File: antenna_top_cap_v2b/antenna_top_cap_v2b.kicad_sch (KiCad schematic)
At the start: 32 parts, among them J1 DEBUG, J12 USB_C_Receptacle_USB2.0_16P, J2 Battery Charge Bypass, J3 FC Reset Jumper, J4 FC USB Bootselect Jumper, J5 Conn_Coaxial, Q1 BSS138, U1 VL6180XV0NR/1, U16 MCP9808T-E/MS, U2 LP5907-2.8V, U4 VEML7700, U5 HHM1591D1

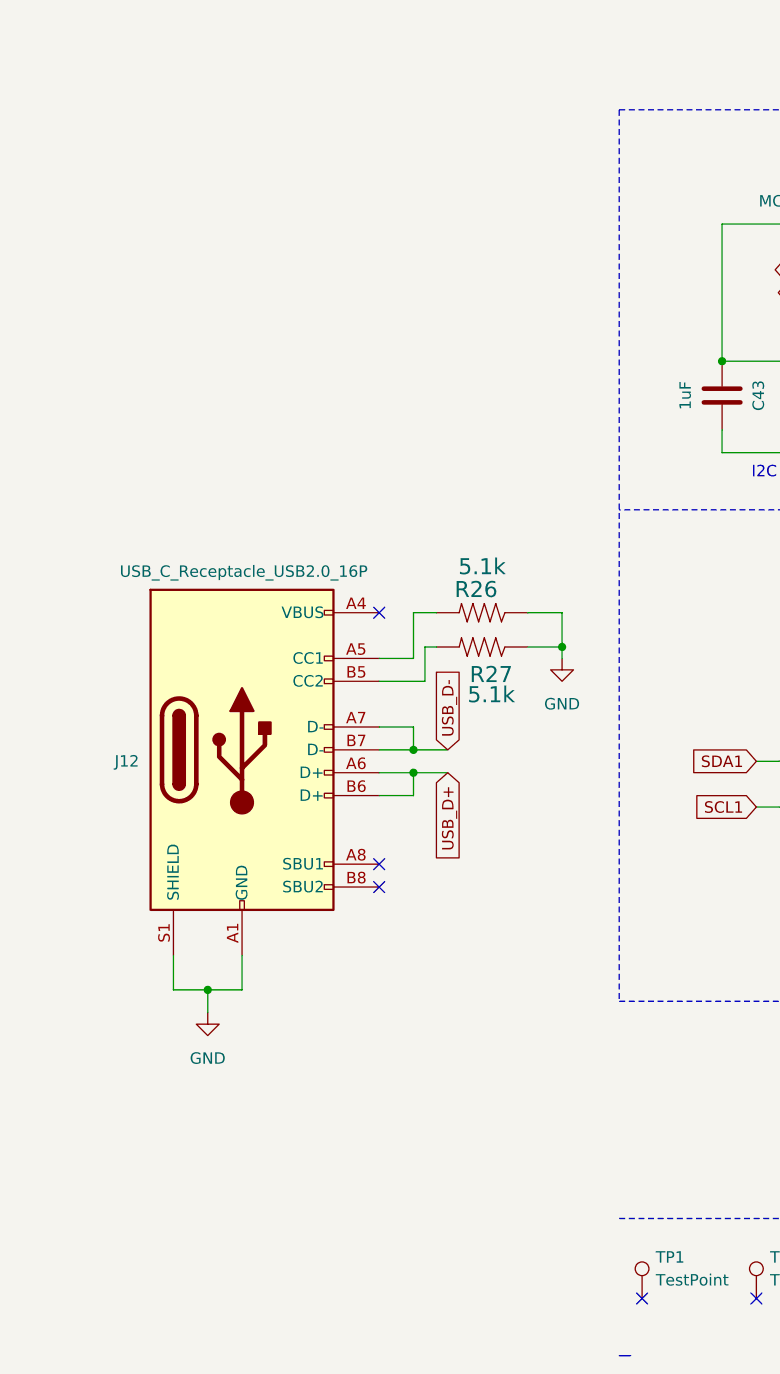
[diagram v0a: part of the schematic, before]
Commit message: Added Payload USB Passthrough
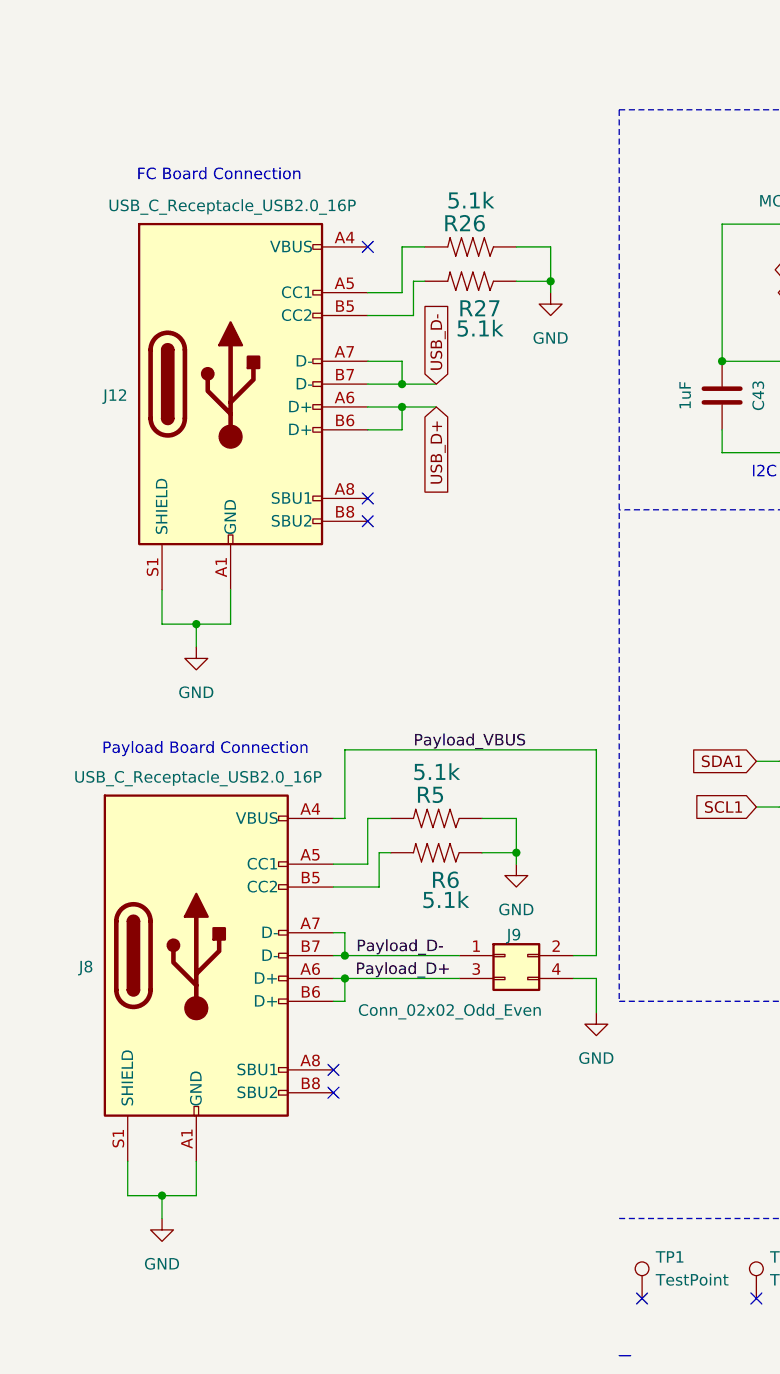
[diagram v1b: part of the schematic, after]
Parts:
- added J8: USB_C_Receptacle_USB2.0_16P, Connector_USB:USB_C_Receptacle_HRO_TYPE-C-31-M-12, symbol Connector:USB_C_Receptacle_USB2.0_16P
- added J9: Conn_02x02_Odd_Even, Connector_Hirose:Hirose_DF11-4DP-2DSA_2x02_P2.00mm_Vertical, symbol Connector_Generic:Conn_02x02_Odd_Even
- added R5, R6: 5.1k, Resistor_SMD:R_0603_1608Metric, symbol mainboard:RESISTOR0603
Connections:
- net GND: now also J8.A1 (GND), J8.A12 (GND), J8.B1 (GND), J8.B12 (GND), J8.S1 (SHIELD), J9.4 (Pin_4), R5.1, R6.1
- new net: J8.A5 (CC1), R5.2
- new net: J8.B5 (CC2), R6.2
- new net Payload_D+: J8.A6 (D+), J8.B6 (D+), J9.3 (Pin_3)
- new net Payload_D-: J8.A7 (D-), J8.B7 (D-), J9.1 (Pin_1)
- new net Payload_VBUS: J8.A4 (VBUS), J8.A9 (VBUS), J8.B4 (VBUS), J8.B9 (VBUS), J9.2 (Pin_2)
- no-connect marks 13 -> 15
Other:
- note added: "FC Board Connection"
- note added: "Payload Board Connection"
- moved on the sheet: J12, R26, R27
